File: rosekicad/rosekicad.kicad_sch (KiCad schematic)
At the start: 4 parts, among them Q1 2N2222

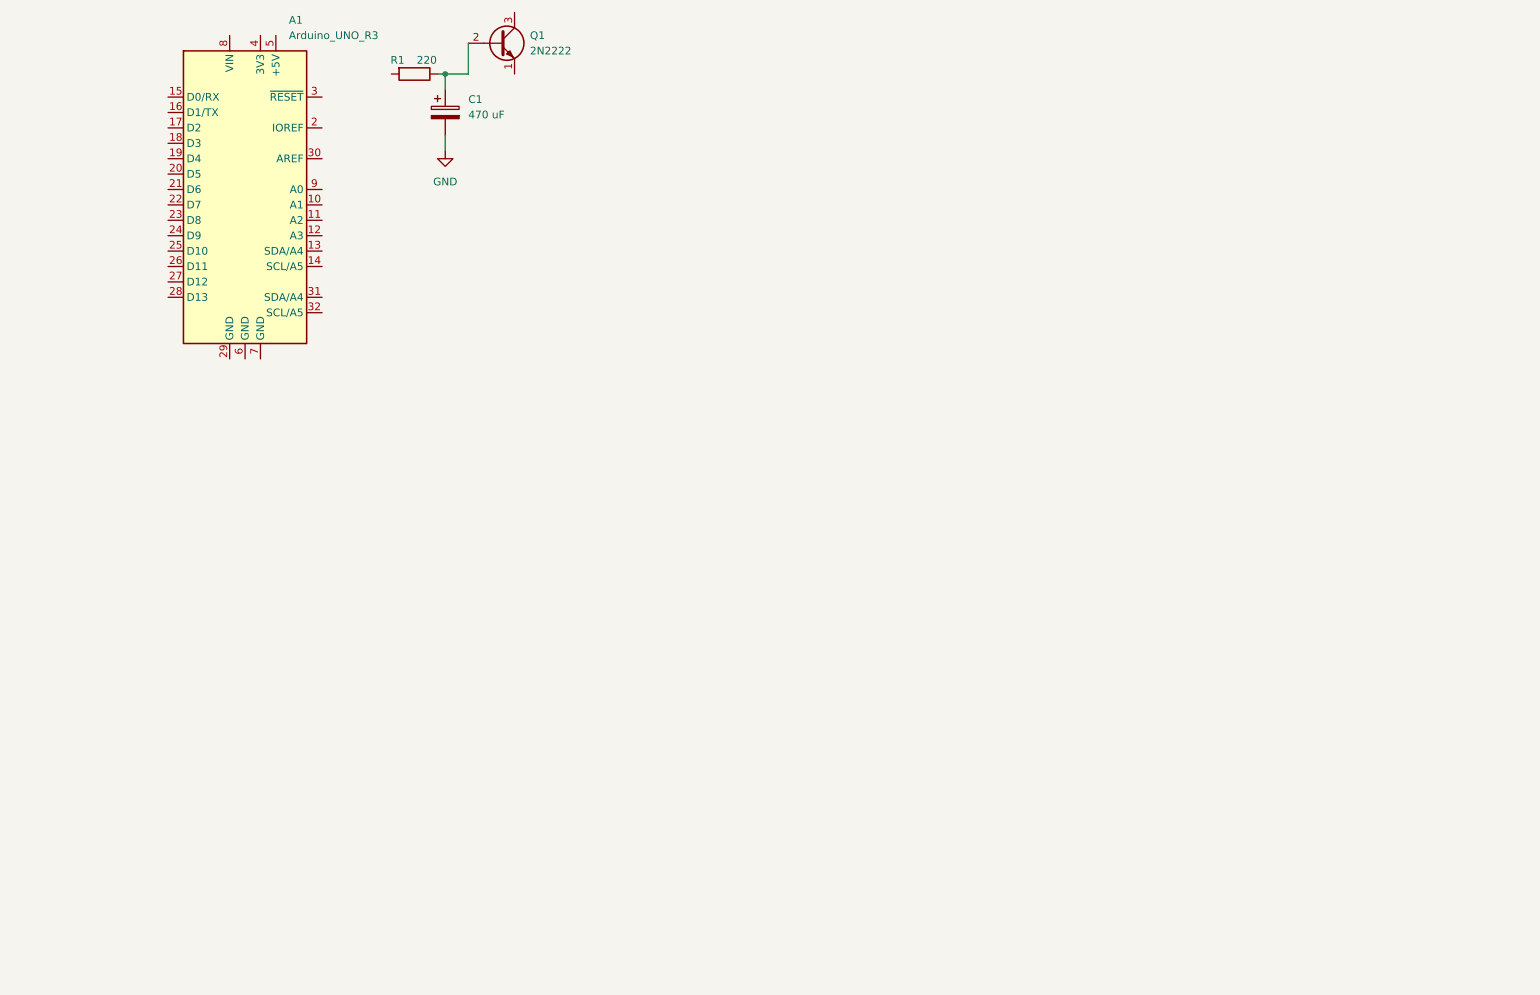
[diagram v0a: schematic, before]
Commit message: updated scheatic
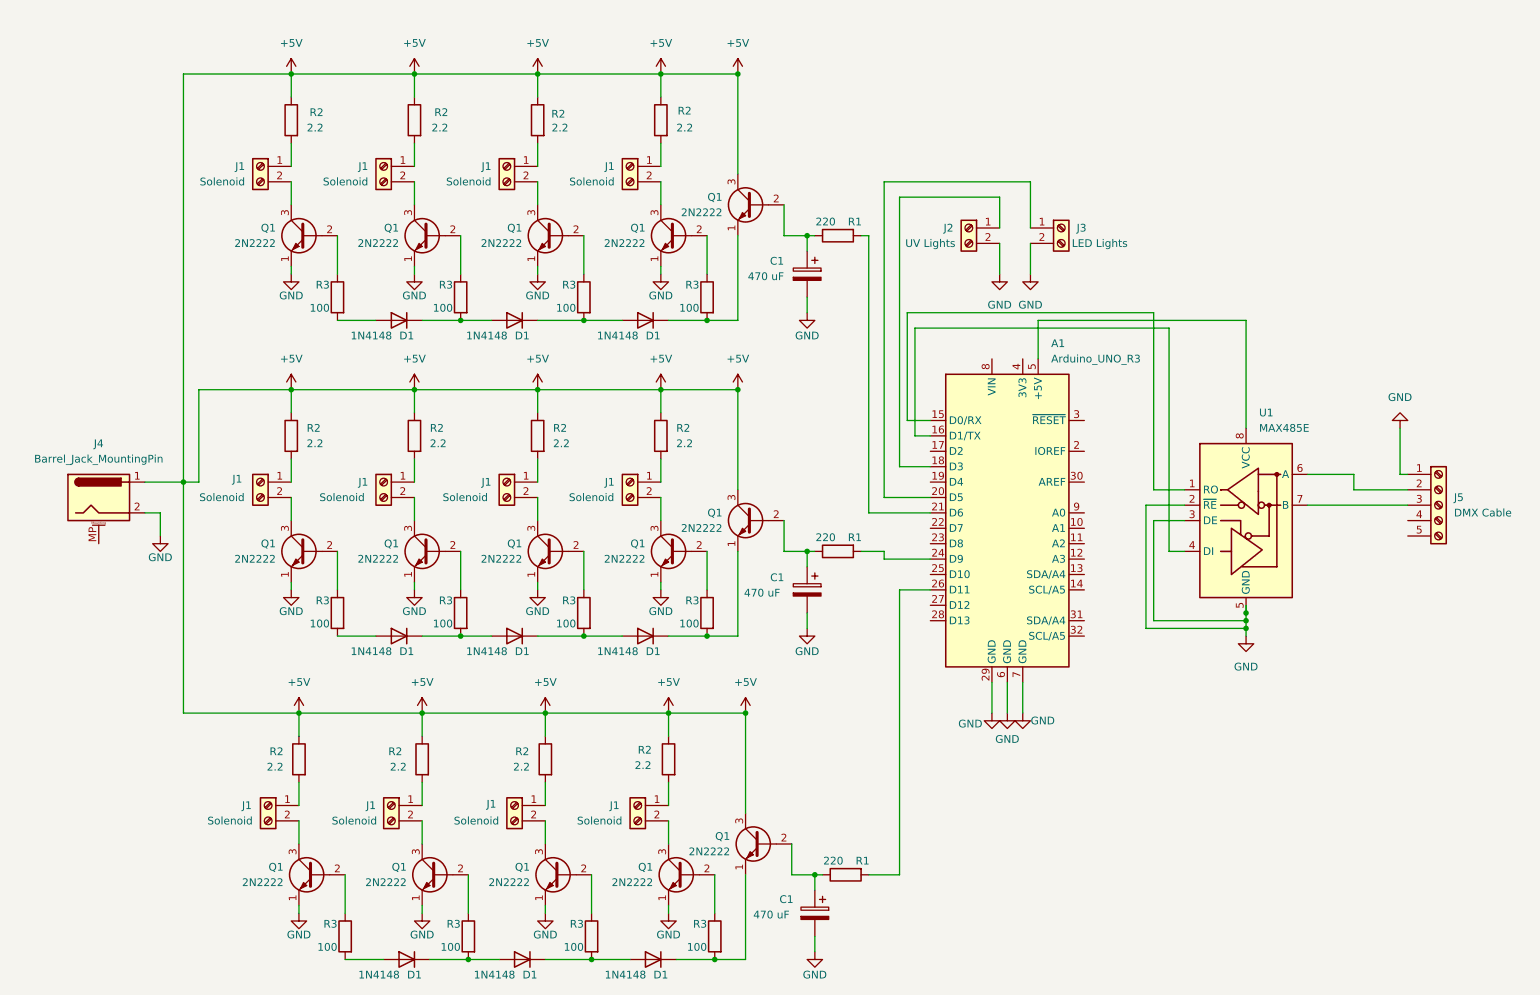
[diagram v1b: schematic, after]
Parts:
- added C1 (x2): 470 uF, symbol Device:C_Polarized
- added D1 (x9): 1N4148, Diode_THT:D_DO-35_SOD27_P7.62mm_Horizontal, symbol Diode:1N4148
- added J1 (x12): Solenoid, symbol Connector:Screw_Terminal_01x02
- added J2: UV Lights, symbol Connector:Screw_Terminal_01x02
- added J3: LED Lights, symbol Connector:Screw_Terminal_01x02
- added J4: Barrel_Jack_MountingPin, symbol Connector:Barrel_Jack_MountingPin
- added J5: DMX Cable, symbol Connector:Screw_Terminal_01x05
- added Q1 (x14): 2N2222, Package_TO_SOT_THT:TO-92_Inline, symbol Transistor_BJT:2N3904
- added R1 (x2): 220, symbol Device:R
- added R2 (x12): 2.2, symbol Device:R
- added R3 (x12): 100, symbol Device:R
- added U1: MAX485E, Package_SO:SOIC-8_3.9x4.9mm_P1.27mm, symbol Interface_UART:MAX485E
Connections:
- net GND: now also A1.29 (GND), A1.6 (GND), A1.7 (GND), C1.2, C1.2, J2.2 (Pin_2), J3.2 (Pin_2), J4.2, J5.1 (Pin_1), Q1.1 (E), Q1.1 (E), Q1.1 (E), Q1.1 (E), Q1.1 (E), Q1.1 (E), Q1.1 (E), Q1.1 (E), Q1.1 (E), Q1.1 (E), Q1.1 (E), Q1.1 (E), U1.2 (~{RE}), U1.3 (DE), U1.5 (GND)
- net at Q1.1 (E): now also D1.1 (K), R3.2
- net +5V: now reaches Q1.3 (C)
- net +5V: now also J4.1, Q1.3 (C), Q1.3 (C), R2.1, R2.1, R2.1, R2.1, R2.1, R2.1, R2.1, R2.1, R2.1, R2.1, R2.1, R2.1
- net at R1.2: now also A1.21 (D6)
- net at A1.15 (D0/RX): now also U1.1 (RO)
- net at A1.16 (D1/TX): now also U1.4 (DI)
- net at A1.18 (D3): now also J2.1 (Pin_1)
- net at A1.20 (D5): now also J3.1 (Pin_1)
- net at A1.24 (D9): now also R1.2
- net at A1.26 (D11): now also R1.2
- net at A1.5 (+5V): now also U1.8 (VCC)
- new net: J1.1 (Pin_1), R2.2 (x12)
- new net: Q1.2 (B), R3.1 (x12)
- new net: D1.1 (K), D1.2 (A), R3.2 (x6)
- new net: D1.1 (K), Q1.1 (E), R3.2 (x2)
- new net: D1.2 (A), R3.2 (x3)
- new net: J1.2 (Pin_2), Q1.3 (C) (x12)
- new net: C1.1, Q1.2 (B), R1.1 (x2)
- new net: J5.2 (Pin_2), U1.6 (A)
- new net: J5.3 (Pin_3), U1.7 (B)
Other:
- company: (none) -> Anna Tretiakova
- title: (none) -> Senior Design Rose
- moved on the sheet: C1, Q1, R1
